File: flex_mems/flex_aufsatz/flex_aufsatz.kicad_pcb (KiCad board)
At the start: 2 copper layers, 11 parts, among them IC1 ADPL44002AUJZ-1.8-R7, J1 Conn_01x22_Socket, J2 Conn_01x22_Socket, J3 10164228-0101A1RLF, J4 10164228-0101A1RLF, U1 ADAU7118ACPZRL

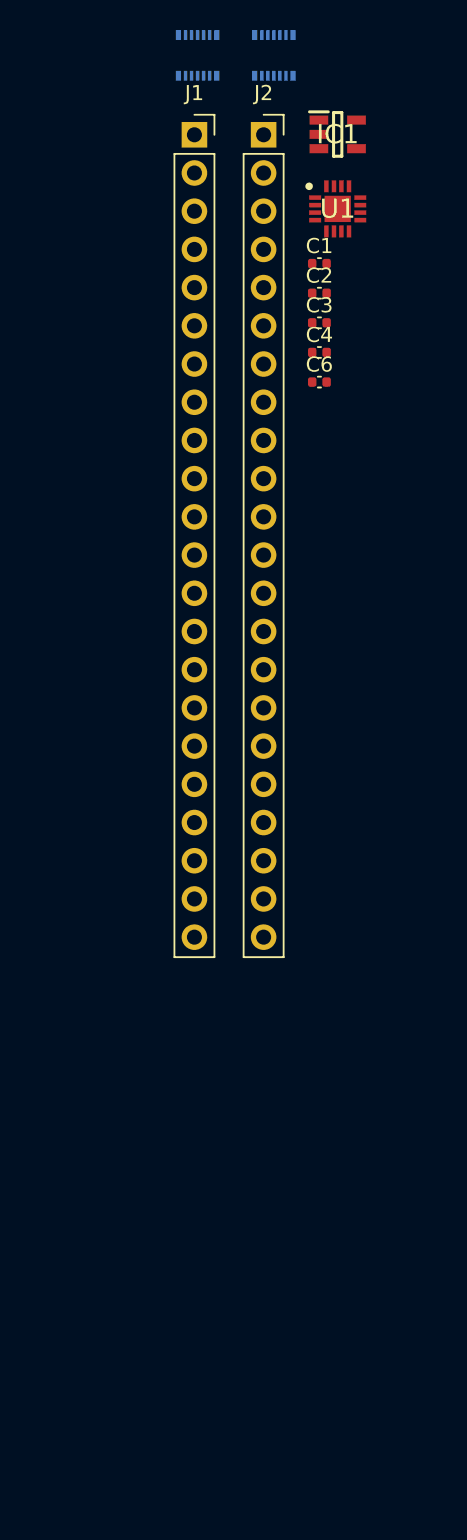
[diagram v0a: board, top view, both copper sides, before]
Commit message: flex_aufsatz1.0
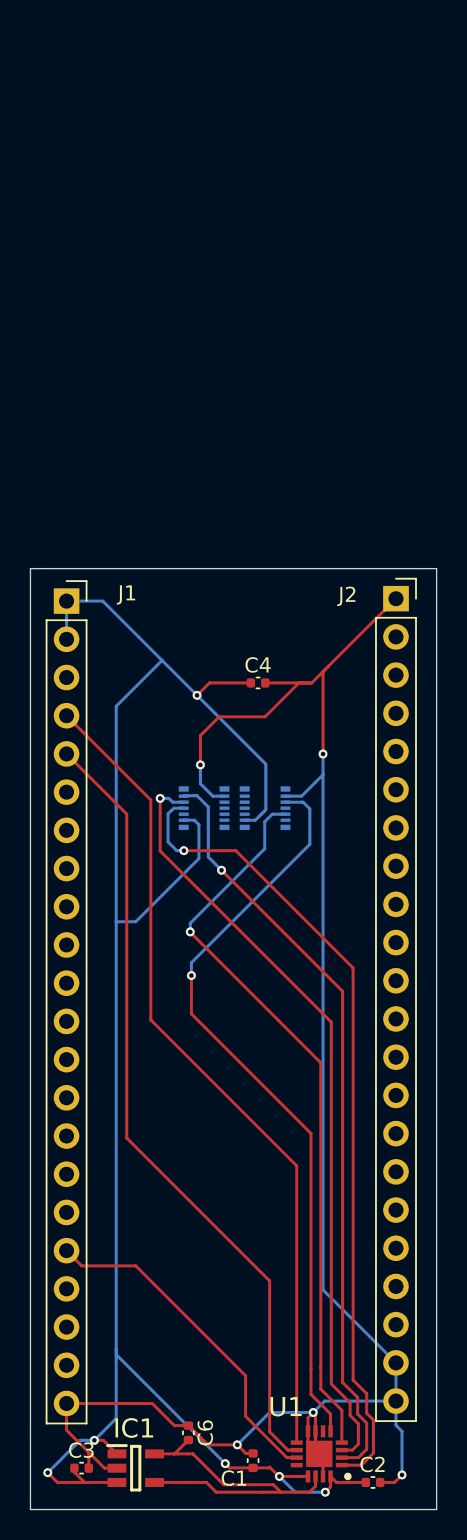
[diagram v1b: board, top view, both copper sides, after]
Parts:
- moved IC1 89.7 mm to (102.0, 157.8)
- moved U1 82.8 mm to (114.2, 156.8), turned to 180 degrees
- moved C1 79.7 mm to (109.8, 157.3), turned to 90 degrees
- moved C2 79.1 mm to (117.8, 158.8)
- moved C3 77.8 mm to (98.4, 157.8)
- moved C6 70.4 mm to (105.5, 155.4), turned to -90 degrees
- moved J4 50.0 mm to (110.6, 113.9), turned to 90 degrees
- moved J3 50.0 mm to (106.5, 113.9), turned to 90 degrees
- moved J1 32.1 mm to (97.4, 100.2)
- moved J2 32.1 mm to (119.3, 100.0)
- moved C4 22.3 mm to (110.1, 105.6)
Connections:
- J1 pad 2: unconnected-(J1-Pin_2-Pad2) -> +3.3V
- J2 pad 21: unconnected-(J2-Pin_21-Pad21) -> GND
- J2 pad 22: unconnected-(J2-Pin_22-Pad22) -> GND
- J3 pad 1: +3V3 -> +3.3V
- J4 pad 1: +3V3 -> +3.3V
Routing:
- net +3.3V: track 0.00 -> 128.0 mm, vias 0 -> 6
- net GND: track 0.00 -> 124.5 mm, vias 0 -> 5
- net /WS: track 0.00 -> 54.7 mm
- net /MIC_CLK0: track 0.00 -> 53.3 mm, vias 0 -> 1
- net /BCLK: track 0.00 -> 53.0 mm
- net /MIC_DOUT_1: track 0.00 -> 50.4 mm, vias 0 -> 1
- net /MIC_DOUT_0: track 0.00 -> 50.2 mm, vias 0 -> 1
- net /MIC_DOUT_2: track 0.00 -> 49.2 mm, vias 0 -> 1
- net /MIC_CLK1: track 0.00 -> 48.2 mm, vias 0 -> 1
- net /TDM_DATA: track 0.00 -> 22.6 mm
- net +1V8: track 0.00 -> 22.6 mm
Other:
- board outline added: 27 x 62.6 mm
